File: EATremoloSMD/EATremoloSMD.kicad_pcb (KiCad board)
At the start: 2 copper layers, 81.8 x 85.1 mm, 40 parts, among them J1 JACK__MONO_2P_NC, J2 BARREL_JACK, J3 JACK__MONO_2P_NC, Q1 Q_NJFET_DSG, Q2 Q_NPN_EBC, Q3 Q_NPN_EBC, Q4 Q_NJFET_DSG, SW1 SW_3PDT_on_on

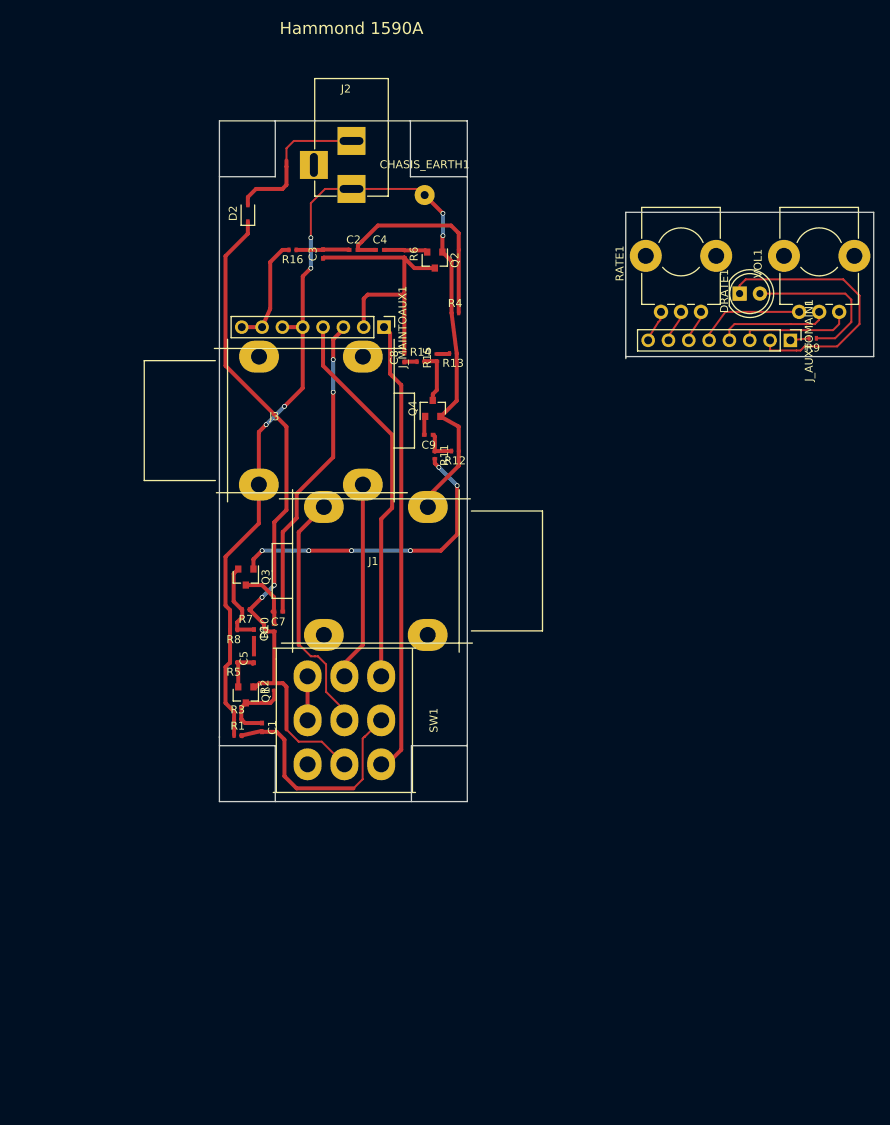
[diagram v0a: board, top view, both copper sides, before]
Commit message: BoardUpdate
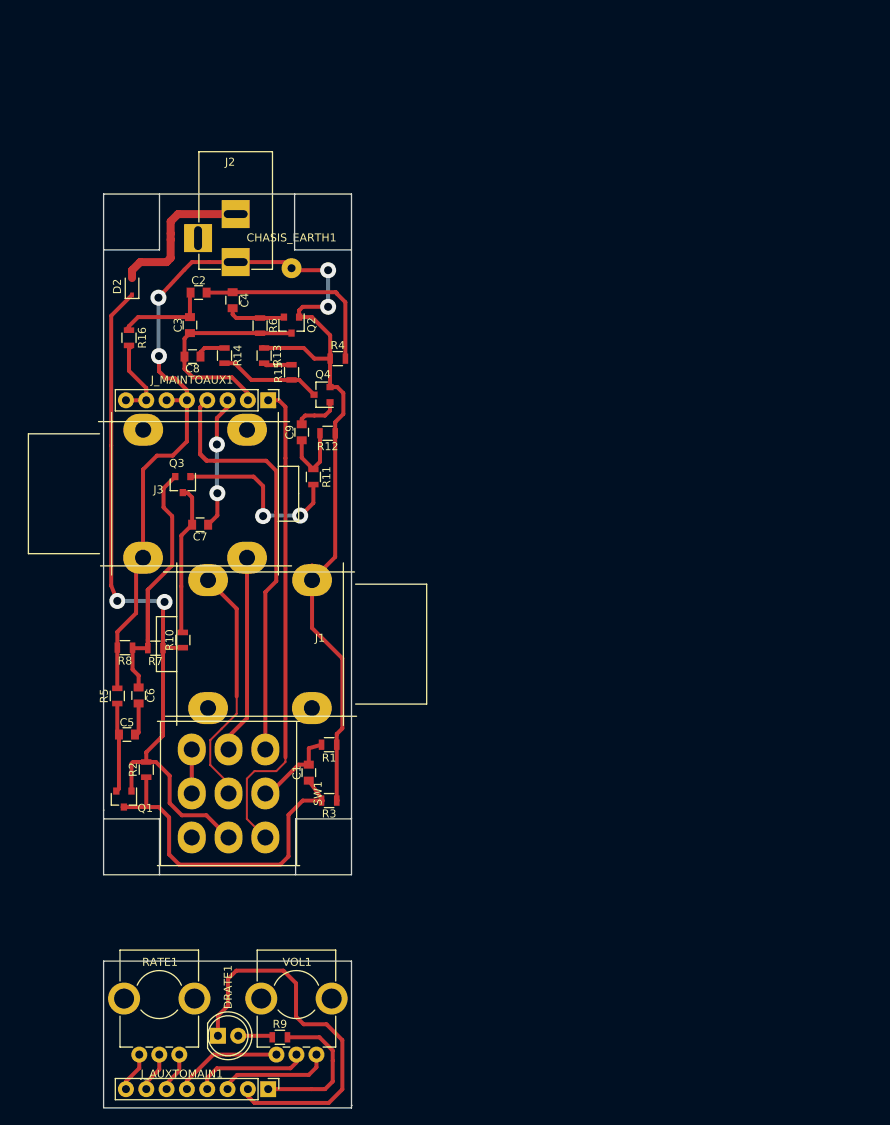
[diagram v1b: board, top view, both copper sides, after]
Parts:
- C1, C2, C3, C4, C5, C6, C7, C8, C9: footprint Capacitors_SMD:C_0402_NoSilk -> Capacitors_SMD:C_0805
- R1, R10, R11, R12, R13, R14, R15, R16, R2, R3, R4, R5, R6, R7, R8, R9: footprint Resistors_SMD:R_0402_NoSilk -> Resistors_SMD:R_0805
- moved J_AUXTOMAIN1 114.1 mm to (108.0, 182.1)
- moved VOL1 113.5 mm to (114.0, 177.8)
- moved RATE1 113.5 mm to (96.8, 177.8)
- moved DRATE1 113.4 mm to (101.7, 175.5)
- moved R9 109.9 mm to (109.4, 175.6), turned to 0 degrees
- moved C8 26.5 mm to (98.5, 90.6), turned to 180 degrees
- moved R14 24.5 mm to (102.5, 90.4), turned to 270 degrees
- moved R13 23.6 mm to (107.4, 90.4), turned to 270 degrees
- moved R16 23.2 mm to (90.6, 88.2), turned to 270 degrees
- moved R6 20.1 mm to (106.9, 86.7)
- moved C2 20.1 mm to (99.3, 82.5)
- moved Q1 20.0 mm to (89.9, 145.9)
- moved Q2 19.7 mm to (110.9, 86.6)
- moved C4 19.5 mm to (103.5, 83.5), turned to 270 degrees
- moved R2 19.1 mm to (92.7, 142.2)
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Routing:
- net /GND: track 134.0 -> 171.1 mm, vias 6 -> 4
- net Net-(C1-Pad1): track 9.93 -> 44.2 mm
- net Net-(C6-Pad1): track 10.7 -> 38.3 mm
- net /VOL_P3: track 38.7 -> 17.0 mm
- net Net-(C1-Pad2): track 29.8 -> 10.6 mm
- net Net-(J_AUXTOMAIN1-Pad1): track 2.36 -> 18.7 mm
- net Net-(Q3-Pad1): track 38.6 -> 22.8 mm, vias 6 -> 2
- net Net-(DRATE1-Pad2): track 19.8 -> 4.34 mm
- net Net-(DRATE1-Pad1): track 34.5 -> 49.4 mm
- net Net-(C7-Pad2): track 7.75 -> 19.2 mm
- net Net-(C5-Pad1): track 5.46 -> 12.0 mm
- net /LED_AN: track 35.4 -> 29.0 mm
- net /VOL_P2: track 47.8 -> 54.0 mm
- net /+9V: track 84.8 -> 91.0 mm
- net Net-(Q4-Pad3): track 6.72 -> 12.8 mm
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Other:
- board size 81.8 x 85.1 mm -> 31.1 x 114.2 mm
- board text removed: "Hammond 1590A"

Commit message: Update
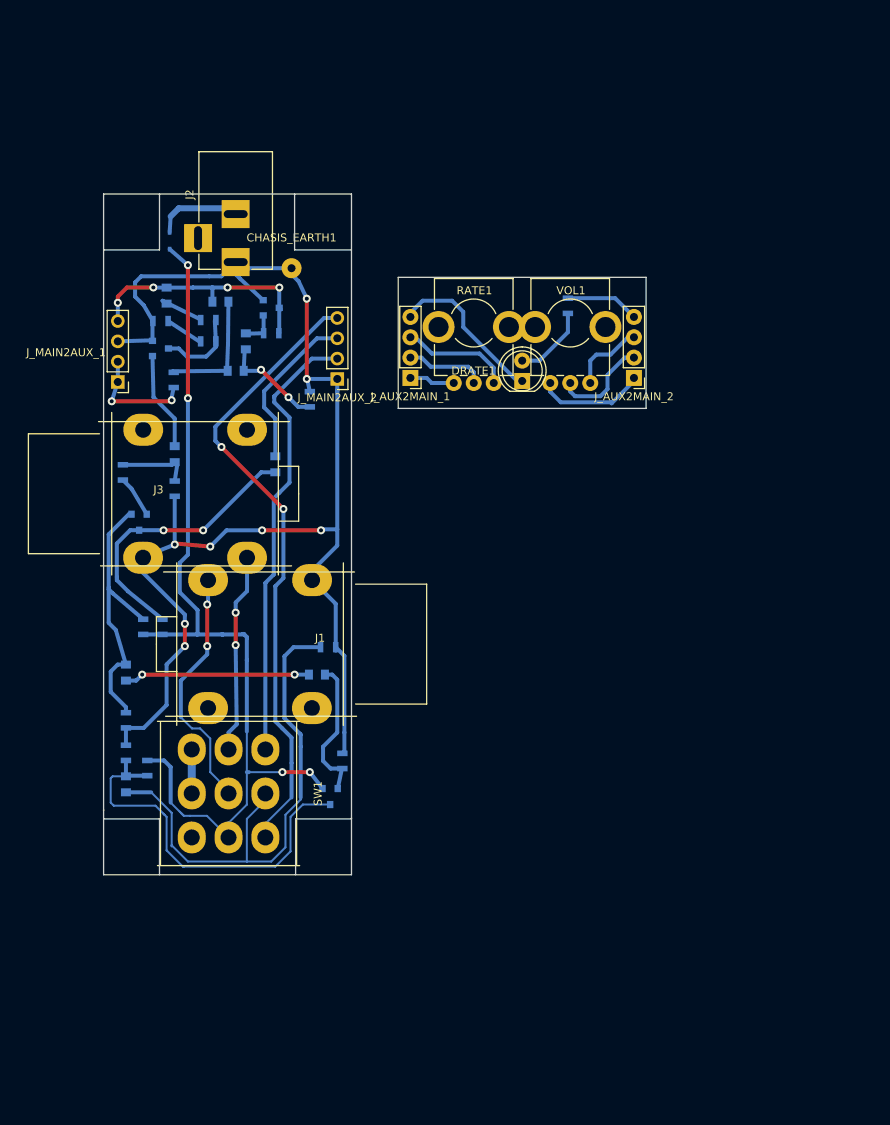
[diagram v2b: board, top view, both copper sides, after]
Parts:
- removed J_AUXTOMAIN1, J_MAINTOAUX1: CONN_01X08, Pin_Headers:Pin_Header_Straight_1x08_Pitch2.54mm
- added J_AUX2MAIN_1: CONN_01X04, Pin_Headers:Pin_Header_Straight_1x04_Pitch2.54mm, F.Cu at (125.7, 93.2)
- added J_AUX2MAIN_2: CONN_01X04, Pin_Headers:Pin_Header_Straight_1x04_Pitch2.54mm, F.Cu at (153.7, 93.2)
- added J_MAIN2AUX_1: CONN_01X04, Pin_Headers:Pin_Header_Straight_1x04_Pitch2.54mm, F.Cu at (89.2, 93.7)
- added J_MAIN2AUX_2: CONN_01X04, Pin_Headers:Pin_Header_Straight_1x04_Pitch2.54mm, F.Cu at (116.6, 93.3)
- C1, C2, C3, C4, C5, C6, C7, C8, C9, D2, Q1, Q2, Q3, Q4, R1, R10, R11, R12, R13, R14, R15, R2, R3, R4, R5, R6, R7, R8, R9: moved to B.Cu
- R16: value 1K -> 4K7; moved to B.Cu
- moved R9 98.3 mm to (145.4, 84.2), turned to 90 degrees
- moved RATE1 92.7 mm to (136.1, 93.9)
- moved VOL1 90.7 mm to (148.2, 93.9)
- moved DRATE1 90.3 mm to (139.7, 93.6), turned to 90 degrees
- moved R5 29.3 mm to (117.2, 141.1)
- moved R3 26.1 mm to (90.2, 140.1), turned to 270 degrees
- moved Q1 25.8 mm to (115.7, 145.5)
- moved C5 24.9 mm to (114.0, 130.3), turned to 180 degrees
- moved R11 23.8 mm to (89.8, 105.0)
- moved C1 22.9 mm to (90.2, 144.0), turned to 270 degrees
- moved Q4 21.0 mm to (94.5, 89.5), turned to 0 degrees
- moved R12 20.3 mm to (96.3, 107.1), turned to 90 degrees
- moved C9 16.1 mm to (96.3, 102.7)
- moved R13 13.7 mm to (94.5, 86.1), turned to 0 degrees
- moved R1 12.2 mm to (115.4, 126.9)
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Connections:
- C3 pad 1: /LED_AN -> /LED_CA
- C8 pad 2: /LED_AN -> /LED_CA
- Q2 pad 1: /GND -> Net-(C4-Pad2)
- Q2 pad 2: Net-(C4-Pad2) -> /GND
- Q2 pad 3: /LED_AN -> /LED_CA
- Q3 pad 1: Net-(Q3-Pad1) -> Net-(C6-Pad1)
- Q3 pad 2: Net-(C6-Pad1) -> Net-(Q3-Pad2)
- R11 pad 2: Net-(Q3-Pad1) -> Net-(Q3-Pad2)
- R6 pad 2: /LED_AN -> /LED_CA
- SW1 pad 3: /LED_CA -> /LED_AN
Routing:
- net Net-(C1-Pad2): track 10.6 -> 66.9 mm
- net /LED_AN: track 29.0 -> 78.4 mm, vias 0 -> 2
- net /LED_CA: track 62.7 -> 32.1 mm, vias 0 -> 4
- net Net-(DRATE1-Pad1): track 49.4 -> 20.4 mm
- net /+9V: track 91.0 -> 118.3 mm, vias 2 -> 4
- net Net-(Q3-Pad1): track 22.8 -> 0.00 mm, vias 2 -> 0
- net Net-(C5-Pad2): track 4.20 -> 23.2 mm, vias 0 -> 2
- net Net-(C7-Pad2): track 19.2 -> 35.6 mm, vias 0 -> 2
- net Net-(C2-Pad2): track 25.0 -> 13.0 mm, vias 0 -> 2
- net Net-(J_AUX2MAIN_2-Pad4): track 18.7 -> 9.48 mm
- net Net-(D2-Pad2): track 19.9 -> 10.9 mm
- net Net-(J_AUX2MAIN_1-Pad3): track 6.25 -> 13.9 mm
- net Net-(C9-Pad2): track 5.84 -> 12.4 mm
- net Net-(C5-Pad1): track 12.0 -> 18.3 mm
- net Net-(Q3-Pad2): track 0.00 -> 5.24 mm
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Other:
- board size 31.1 x 114.2 mm -> 67.8 x 85.1 mm
